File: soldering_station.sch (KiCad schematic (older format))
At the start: 70 parts, among them IC1 ATMEGA8A-P, P1 17v, P2 220v, P3 24v|220v, P4 solder, P5 thermocouple, P6 Fan, P7 thermocouple, P8 Heater, Q1 КТ313Б, Q2 КТ313Б, Q3 КТ313Б, Q4 КТ815А, SW1 mode, SW2 Enc, U1 TL072, U2 MOC3023M, U3 MOC3023M, U4 LM7805CT

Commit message: Fix board
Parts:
- BZ1: symbol Buzzer -> soldering_station-rescue:Buzzer
- C1, C2, C4, C5, C7, C8, C9: symbol C_Small -> soldering_station-rescue:C_Small
- C3, C6: symbol CP_Small -> soldering_station-rescue:CP_Small
- D1, D2: symbol LED -> soldering_station-rescue:LED
- D3, D4: symbol D -> soldering_station-rescue:D
- D5: symbol D_Bridge_+-AA -> soldering_station-rescue:D_Bridge_+-AA
- HG1: symbol ИБ -> иб:ИБ
- HG2, HG3: symbol АЛС324Б1 -> алс324б1:АЛС324Б1
- IC1: symbol ATMEGA8A-P -> atmel:ATMEGA8A-P
- P1, P2, P3, P4, P5, P6, P8: symbol CONN_01X02 -> soldering_station-rescue:CONN_01X02
- P7: symbol CONN_01X03 -> soldering_station-rescue:CONN_01X03
- Q1, Q2, Q3: symbol Q_PNP_CBE -> soldering_station-rescue:Q_PNP_CBE
- Q4: symbol Q_NPN_BCE -> soldering_station-rescue:Q_NPN_BCE
- R1, R10, R11, R12, R13, R14, R15, R16, R17, R18, R19, R2, R20, R21, R22, R23, R24, R25, R26, R27, R28, R3, R4, R5, R6, R7, R8, R9: symbol R -> soldering_station-rescue:R
- RV1, RV2: symbol POT -> soldering_station-rescue:POT
- SB1: symbol Switch -> switch:Switch
- SW1: symbol SW_PUSH -> device:SW_PUSH
- SW2: symbol Rotary_Encoder_Switch -> soldering_station-rescue:Rotary_Encoder_Switch
- U1: symbol TL072 -> soldering_station-rescue:TL072
- U2, U3: symbol MOC3023M -> soldering_station-rescue:MOC3023M
- U4: symbol LM7805CT -> soldering_station-rescue:LM7805CT
- VD1, VD2: symbol BT139 -> bt139:BT139
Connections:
- wire segments 220 -> 260

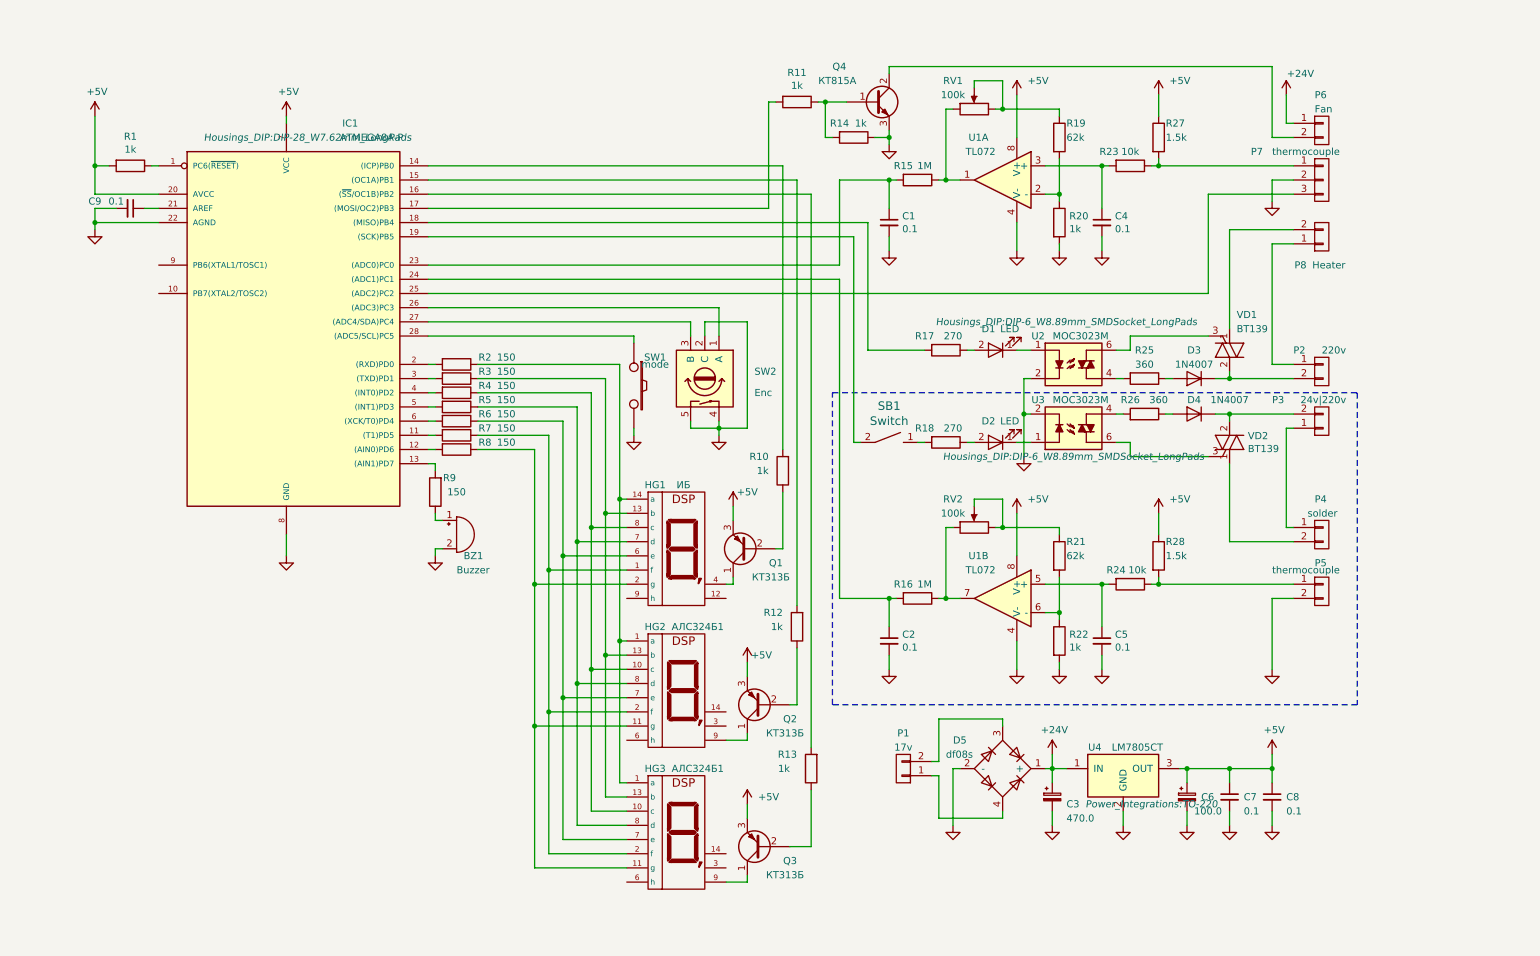
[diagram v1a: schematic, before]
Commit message: Add connectors
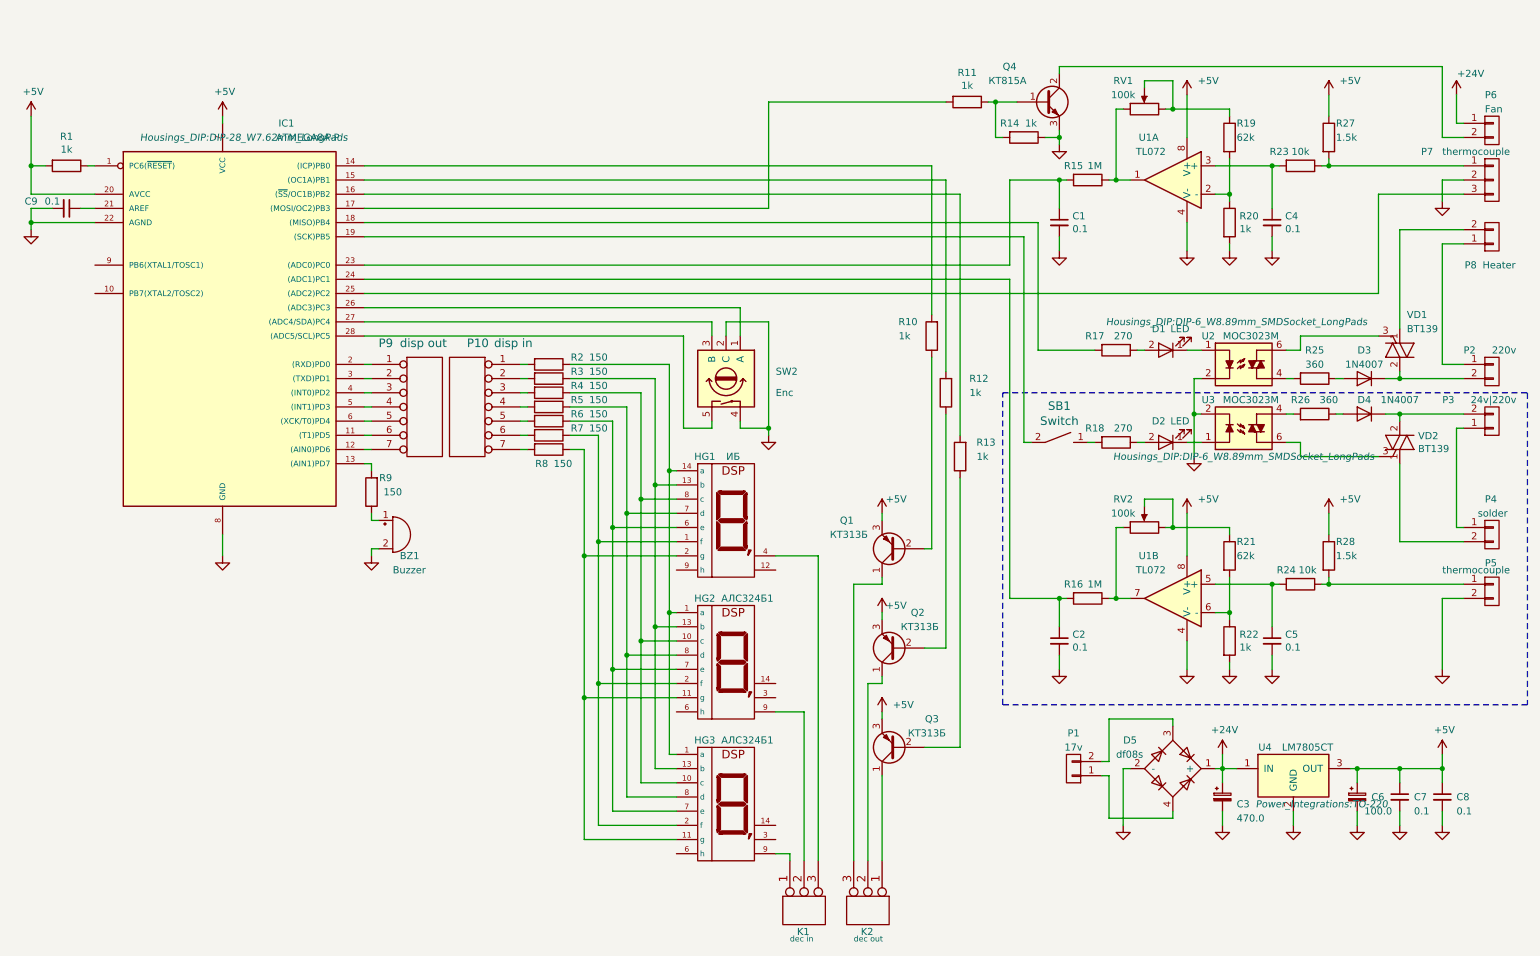
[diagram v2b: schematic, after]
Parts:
- removed SW1: mode, Buttons_Switches_THT:SW_PUSH-12mm, symbol device:SW_PUSH
- added K1: dec in, Pin_Headers:Pin_Header_Straight_1x03_Pitch2.54mm, symbol conn:CONN_3
- added K2: dec out, Pin_Headers:Pin_Header_Straight_1x03_Pitch2.54mm, symbol conn:CONN_3
- added P10: disp in, Pin_Headers:Pin_Header_Straight_1x07_Pitch2.54mm, symbol conn:CONN_7
- added P9: disp out, Pin_Headers:Pin_Header_Straight_1x07_Pitch2.54mm, symbol conn:CONN_7
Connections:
- net GND: no longer SW2.5
- net at IC1.11 ((T1)PD5): now also P9.6 (P6); no longer R7.2
- net at IC1.12 ((AIN0)PD6): now also P9.7 (P7); no longer R8.2
- net at IC1.2 ((RXD)PD0): now also P9.1 (P1); no longer R2.2
- net at IC1.28 ((ADC5/SCL)PC5): now also SW2.5
- net at IC1.3 ((TXD)PD1): now also P9.2 (P2); no longer R3.2
- net at IC1.4 ((INT0)PD2): now also P9.3 (P3); no longer R4.2
- net at IC1.5 ((INT1)PD3): now also P9.4 (P4); no longer R5.2
- net at IC1.6 ((XCK/T0)PD4): now also P9.5 (P5); no longer R6.2
- net at HG2.9: now also K1.2 (PM); no longer Q2.1 (C)
- net at HG3.9: now also K1.1 (P1); no longer Q3.1 (C)
- net at HG1.4: now also K1.3 (P3); no longer Q1.1 (C)
- new net: P10.1 (P1), R2.2
- new net: P10.2 (P2), R3.2
- new net: P10.6 (P6), R7.2
- new net: P10.3 (P3), R4.2
- new net: P10.4 (P4), R5.2
- new net: P10.5 (P5), R6.2
- new net: P10.7 (P7), R8.2
- new net: K2.3 (P3), Q1.1 (C)
- new net: K2.2 (PM), Q2.1 (C)
- new net: K2.1 (P1), Q3.1 (C)
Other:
- moved on the sheet: BZ1, C1, C2, C3, C4, C5, C6, C7, C8, C9, D1, D2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

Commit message: Change triac
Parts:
- removed D3, D4: 1N4007, Diodes_THT:D_5W_P5.08mm_Vertical_AnodeUp, symbol soldering_station-rescue:D
- BZ1: symbol soldering_station-rescue:Buzzer -> soldering_station-rescue:Buzzer-soldering_station-rescue
- C3, C6: symbol soldering_station-rescue:CP_Small -> soldering_station-rescue:CP_Small-soldering_station-rescue
- D1, D2: symbol soldering_station-rescue:LED -> soldering_station-rescue:LED-soldering_station-rescue
- D5: symbol soldering_station-rescue:D_Bridge_+-AA -> soldering_station-rescue:D_Bridge_+-AA-soldering_station-rescue
- HG1: symbol иб:ИБ -> soldering_station-rescue:ИБ-иб
- HG2, HG3: symbol алс324б1:АЛС324Б1 -> soldering_station-rescue:АЛС324Б1-алс324б1
- IC1: symbol atmel:ATMEGA8A-P -> soldering_station-rescue:ATMEGA8A-P-atmel
- K1, K2: symbol conn:CONN_3 -> soldering_station-rescue:CONN_3-conn
- P1, P2, P3, P4, P5, P6, P8: symbol soldering_station-rescue:CONN_01X02 -> soldering_station-rescue:CONN_01X02-soldering_station-rescue
- P10, P9: symbol conn:CONN_7 -> soldering_station-rescue:CONN_7-conn
- P7: symbol soldering_station-rescue:CONN_01X03 -> soldering_station-rescue:CONN_01X03-soldering_station-rescue
- Q1, Q2, Q3: symbol soldering_station-rescue:Q_PNP_CBE -> soldering_station-rescue:Q_PNP_CBE-soldering_station-rescue
- Q4: symbol soldering_station-rescue:Q_NPN_BCE -> soldering_station-rescue:Q_NPN_BCE-soldering_station-rescue
- R25, R26: value 360 -> 270
- SB1: symbol switch:Switch -> soldering_station-rescue:Switch-switch
- SW2: symbol soldering_station-rescue:Rotary_Encoder_Switch -> soldering_station-rescue:Rotary_Encoder_Switch-soldering_station-rescue
- U2, U3: symbol soldering_station-rescue:MOC3023M -> soldering_station-rescue:MOC3023M-soldering_station-rescue
- U4: symbol soldering_station-rescue:LM7805CT -> soldering_station-rescue:LM7805CT-soldering_station-rescue
- VD1, VD2: value BT139 -> BT134; footprint TO_SOT_Packages_THT:TO-220_Vertical -> lib:sot82; symbol bt139:BT139 -> soldering_station-rescue:BT139-bt139
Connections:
- net at R25.1: now also P2.2 (P2), VD1.1 (A1)
- net at R26.1: now also P3.2 (P2), VD2.1 (A1)
- net at VD1.2 (A2): now also P8.2 (P2); no longer P2.2 (P2)
- net at P4.2 (P2): now also VD2.2 (A2); no longer VD2.1 (A1)
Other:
- moved on the sheet: VD1, VD2
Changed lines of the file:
@@
 EESchema Schematic File Version 4
 LIBS:soldering_station-cache
-EELAYER 26 0
+EELAYER 30 0
 EELAYER END
 $Descr A4 11693 8268
@@
 $EndComp
 $Comp
-L atmel:ATMEGA8A-P IC1
+L soldering_station-rescue:ATMEGA8A-P-atmel IC1
 U 1 1 5912C25D
 P 1950 2400
@@
 $EndComp
 $Comp
-L soldering_station-rescue:Buzzer BZ1
+L soldering_station-rescue:Buzzer-soldering_station-rescue BZ1
 U 1 1 5913130E
 P 3150 3900
@@
 $EndComp
 $Comp
-L soldering_station-rescue:MOC3023M U2
+L soldering_station-rescue:MOC3023M-soldering_station-rescue U2
 U 1 1 59143D58
 P 9150 2700
@@
 $EndComp
 $Comp
-L soldering_station-rescue:MOC3023M U3
+L soldering_station-rescue:MOC3023M-soldering_station-rescue U3
 U 1 1 59143E30
 P 9150 3150
@@
 P 9650 2800
 F 0 "R25" V 9450 2800 50  0000 C CNN
-F 1 "360" V 9550 2800 50  0000 C CNN
+F 1 "270" V 9550 2800 50  0000 C CNN
 F 2 "Resistors_SMD:R_0805" V 9580 2800 50  0001 C CNN
 F 3 "" H 9650 2800 50  0000 C CNN
@@
 P 9650 3050
 F 0 "R26" V 9750 2950 50  0000 C CNN
-F 1 "360" V 9750 3150 50  0000 C CNN
+F 1 "270" V 9750 3150 50  0000 C CNN
 F 2 "Resistors_SMD:R_0805" V 9580 3050 50  0001 C CNN
 F 3 "" H 9650 3050 50  0000 C CNN
@@
 $EndComp
 $Comp
-L soldering_station-rescue:D D3
-U 1 1 591456C9
-P 10000 2800
-F 0 "D3" H 10000 2600 50  0000 C CNN
-F 1 "1N4007" H 10000 2700 50  0000 C CNN
-F 2 "Diodes_THT:D_5W_P5.08mm_Vertical_AnodeUp" H 10000 2800 50  0001 C CNN
-F 3 "" H 10000 2800 50  0000 C CNN
-	1    10000 2800
-	-1   0    0    1
-$EndComp
-$Comp
-L bt139:BT139 VD1
+L soldering_station-rescue:BT139-bt139 VD1
 U 1 1 59145DE9
-P 10250 2600
-F 0 "VD1" H 10300 2350 50  0000 L CNN
-F 1 "BT139" H 10300 2450 50  0000 L CNN
-F 2 "TO_SOT_Packages_THT:TO-220_Vertical" V 10325 2625 50  0001 C CNN
-F 3 "" V 10250 2600 50  0000 C CNN
-	1    10250 2600
+P 10250 2500
+F 0 "VD1" H 10300 2250 50  0000 L CNN
+F 1 "BT134" H 10300 2350 50  0000 L CNN
+F 2 "lib:sot82" V 10325 2525 50  0001 C CNN
+F 3 "" V 10250 2500 50  0000 C CNN
+	1    10250 2500
+	1    0    0    -1
+$EndComp
+$Comp
+L soldering_station-rescue:BT139-bt139 VD2
+U 1 1 59145E5D
+P 10250 3350
+F 0 "VD2" H 10379 3396 50  0000 L CNN
+F 1 "BT134" H 10379 3305 50  0000 L CNN
+F 2 "lib:sot82" V 10325 3375 50  0001 C CNN
+F 3 "" V 10250 3350 50  0000 C CNN
+	1    10250 3350
 	1    0    0    1
-$EndComp
-$Comp
-L bt139:BT139 VD2
-U 1 1 59145E5D
-P 10250 3250
-F 0 "VD2" H 10379 3296 50  0000 L CNN
-F 1 "BT139" H 10379 3205 50  0000 L CNN
-F 2 "TO_SOT_Packages_THT:TO-220_Vertical" V 10325 3275 50  0001 C CNN
-F 3 "" V 10250 3250 50  0000 C CNN
-	1    10250 3250
-	1    0    0    -1
-$EndComp
-$Comp
-L soldering_station-rescue:D D4
-U 1 1 5914649B
-P 10000 3050
-F 0 "D4" H 10000 3150 50  0000 C CNN
-F 1 "1N4007" H 9750 3150 50  0000 C CNN
-F 2 "Diodes_THT:D_5W_P5.08mm_Vertical_AnodeUp" H 10000 3050 50  0001 C CNN
-F 3 "" H 10000 3050 50  0000 C CNN
-	1    10000 3050
-	-1   0    0    -1
 $EndComp
 $Comp
@@
 $EndComp
 $Comp
-L soldering_station-rescue:LED D1
+L soldering_station-rescue:LED-soldering_station-rescue D1
 U 1 1 59146F29
 P 8600 2600
@@
 $EndComp
 $Comp
-L soldering_station-rescue:LED D2
+L soldering_station-rescue:LED-soldering_station-rescue D2
 U 1 1 59147091
 P 8600 3250
@@
 $EndComp
 $Comp
-L soldering_station-rescue:CONN_01X02 P2
+L soldering_station-rescue:CONN_01X02-soldering_station-rescue P2
 U 1 1 5914C58F
 P 10900 2750
@@
 $EndComp
 $Comp
-L soldering_station-rescue:CONN_01X02 P3
+L soldering_station-rescue:CONN_01X02-soldering_station-rescue P3
 U 1 1 5914D402
 P 10900 3100
@@
 $EndComp
 $Comp
-L switch:Switch SB1
+L soldering_station-rescue:Switch-switch SB1
 U 1 1 5914E255
 P 7850 3250
@@
 $EndComp
 $Comp
-L soldering_station-rescue:CONN_01X02 P4
+L soldering_station-rescue:CONN_01X02-soldering_station-rescue P4
 U 1 1 5914FDDB
 P 10900 3900
@@
 $EndComp
 $Comp
-L soldering_station-rescue:CONN_01X02 P5
+L soldering_station-rescue:CONN_01X02-soldering_station-rescue P5
 U 1 1 5914FEAB
 P 10900 4300
@@
 $EndComp
 $Comp
-L soldering_station-rescue:Q_NPN_BCE Q4
+L soldering_station-rescue:Q_NPN_BCE-soldering_station-rescue Q4
 U 1 1 5916DF03
 P 7750 850
@@
 $EndComp
 $Comp
-L soldering_station-rescue:LM7805CT U4
+L soldering_station-rescue:LM7805CT-soldering_station-rescue U4
 U 1 1 5916F3BD
 P 9500 5600
@@
 $EndComp
 $Comp
-L soldering_station-rescue:CP_Small C6
+L soldering_station-rescue:CP_Small-soldering_station-rescue C6
 U 1 1 5916FF84
 P 9950 5750
@@
 $EndComp
 $Comp
-L soldering_station-rescue:CP_Small C3
+L soldering_station-rescue:CP_Small-soldering_station-rescue C3
 U 1 1 591704BF
 P 9000 5750
@@
 $EndComp
 $Comp
-L алс324б1:АЛС324Б1 HG2
+L soldering_station-rescue:АЛС324Б1-алс324б1 HG2
 U 1 1 5919A435
 P 5550 4800
@@
 $EndComp
 $Comp
-L алс324б1:АЛС324Б1 HG3
+L soldering_station-rescue:АЛС324Б1-алс324б1 HG3
 U 1 1 5919A4F5
 P 5550 5800
@@
 $EndComp
 $Comp
-L иб:ИБ HG1
+L soldering_station-rescue:ИБ-иб HG1
 U 1 1 5919A59F
 P 5550 3800
@@
 $EndComp
 $Comp
-L soldering_station-rescue:Q_PNP_CBE Q1
+L soldering_station-rescue:Q_PNP_CBE-soldering_station-rescue Q1
 U 1 1 591A31E1
 P 6700 4000
@@
 $EndComp
 $Comp
-L soldering_station-rescue:Q_PNP_CBE Q2
+L soldering_station-rescue:Q_PNP_CBE-soldering_station-rescue Q2
 U 1 1 591A32AD
 P 6700 4700
@@
 $EndComp
 $Comp
-L soldering_station-rescue:Q_PNP_CBE Q3
+L soldering_station-rescue:Q_PNP_CBE-soldering_station-rescue Q3
 U 1 1 591A334F
 P 6700 5400
@@
 $EndComp
 $Comp
-L soldering_station-rescue:D_Bridge_+-AA D5
+L soldering_station-rescue:D_Bridge_+-AA-soldering_station-rescue D5
 U 1 1 591D2084
 P 8650 5550
@@
 $EndComp
 $Comp
-L soldering_station-rescue:CONN_01X02 P1
+L soldering_station-rescue:CONN_01X02-soldering_station-rescue P1
 U 1 1 591D2FEC
 P 7950 5550
@@
 $EndComp
 $Comp
-L soldering_station-rescue:CONN_01X02 P6
+L soldering_station-rescue:CONN_01X02-soldering_station-rescue P6
 U 1 1 5922F5D6
 P 10900 1050
@@
 $EndComp
 $Comp
-L soldering_station-rescue:CONN_01X02 P8
+L soldering_station-rescue:CONN_01X02-soldering_station-rescue P8
 U 1 1 5922F6D0
 P 10900 1800
@@
 $EndComp
 $Comp
-L soldering_station-rescue:CONN_01X03 P7
+L soldering_station-rescue:CONN_01X03-soldering_station-rescue P7
 U 1 1 5922F790
 P 10900 1400
@@
 $EndComp
 $Comp
-L soldering_station-rescue:Rotary_Encoder_Switch SW2
+L soldering_station-rescue:Rotary_Encoder_Switch-soldering_station-rescue SW2
 U 1 1 59883EF1
 P 5500 2800
@@
 	9450 3050 9500 3050
 Wire Wire Line
-	9800 3050 9850 3050
-Wire Wire Line
 	9450 2800 9500 2800
 Wire Wire Line
-	9800 2800 9850 2800
-Wire Wire Line
-	10150 2800 10250 2800
-Wire Wire Line
-	10250 2800 10250 2750
-Wire Wire Line
-	10250 3100 10250 3050
-Wire Wire Line
-	10150 3050 10250 3050
-Wire Wire Line
-	10100 2500 9550 2500
-Wire Wire Line
-	9550 2500 9550 2600
-Wire Wire Line
-	9550 2600 9450 2600
-Wire Wire Line
-	10100 3350 9550 3350
-Wire Wire Line
-	9550 3350 9550 3250
-Wire Wire Line
-	9550 3250 9450 3250
+	10250 2800 10250 2650
+Wire Wire Line
+	10250 3200 10250 3050
 Wire Wire Line
 	8850 2800 8800 2800
@@
 	10550 4350 10550 4850
 Wire Wire Line
-	10250 1750 10250 2450
+	10250 1750 10250 2350
 Wire Wire Line
 	10700 4350 10550 4350
@@
 	10650 3850 10700 3850
 Wire Wire Line
-	10250 3950 10250 3400
+	10250 3950 10250 3500
 Wire Wire Line
 	8100 3250 8050 3250
@@
 	6950 1300 2950 1300
 $Comp
-L conn:CONN_3 K2
+L soldering_station-rescue:CONN_3-conn K2
 U 1 1 5DE2CB58
 P 6500 6550
@@
 	6600 4250 6600 4200
 $Comp
-L conn:CONN_3 K1
+L soldering_station-rescue:CONN_3-conn K1
 U 1 1 5DE67BB4
 P 6050 6550
@@
 	5950 6200 5950 6150
 $Comp
-L conn:CONN_7 P10
+L soldering_station-rescue:CONN_7-conn P10
 U 1 1 5DF4D6C2
 P 3700 3000
@@
 	4050 3300 4100 3300
 $Comp
-L conn:CONN_7 P9
+L soldering_station-rescue:CONN_7-conn P9
 U 1 1 5E0351E0
 P 3350 3000
@@
 Wire Wire Line
 	2950 2300 5600 2300
+Wire Wire Line
+	9800 2800 10250 2800
+Wire Wire Line
+	9450 2600 10100 2600
+Wire Wire Line
+	9800 3050 10250 3050
+Wire Wire Line
+	9450 3250 10100 3250
 $EndSCHEMATC
